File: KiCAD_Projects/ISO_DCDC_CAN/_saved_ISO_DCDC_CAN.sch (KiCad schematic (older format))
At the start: 116 parts, among them IC1 PC817, IC2 PC817, IC3 PC817, IC4 PC817, IC5 PC817, P1 CONN_01X01, P10 CONN_01X02, P11 CONN_01X02, P12 CONN_01X01, P13 CONN_01X04, P14 CONN_01X02, P15 CONN_01X02, P16 TST, P17 CONN_01X06, P19 CONN_01X01, P2 CONN_01X01, P20 CONN_01X01, P21 CONN_01X02, P22 CONN_01X01, P23 CONN_01X01, P25 CONN_01X01, P26 CONN_01X01, P3 CONN_01X01, P4 CONN_01X02, P5 CONN_01X02, P6 CONN_01X04, P7 CONN_01X04, P8 CONN_01X01, P9 CONN_01X01, Q1 MOSFET_N, U1 V23076-D3001-D142, U2 V23076-D3001-D142, U3 V23076-D3001-D142, U4 NCP1117ST285T3G, U5 STM32F103_48, U6 ADM3054, U7 ACS758, U8 ACS758, X1 CRYSTAL

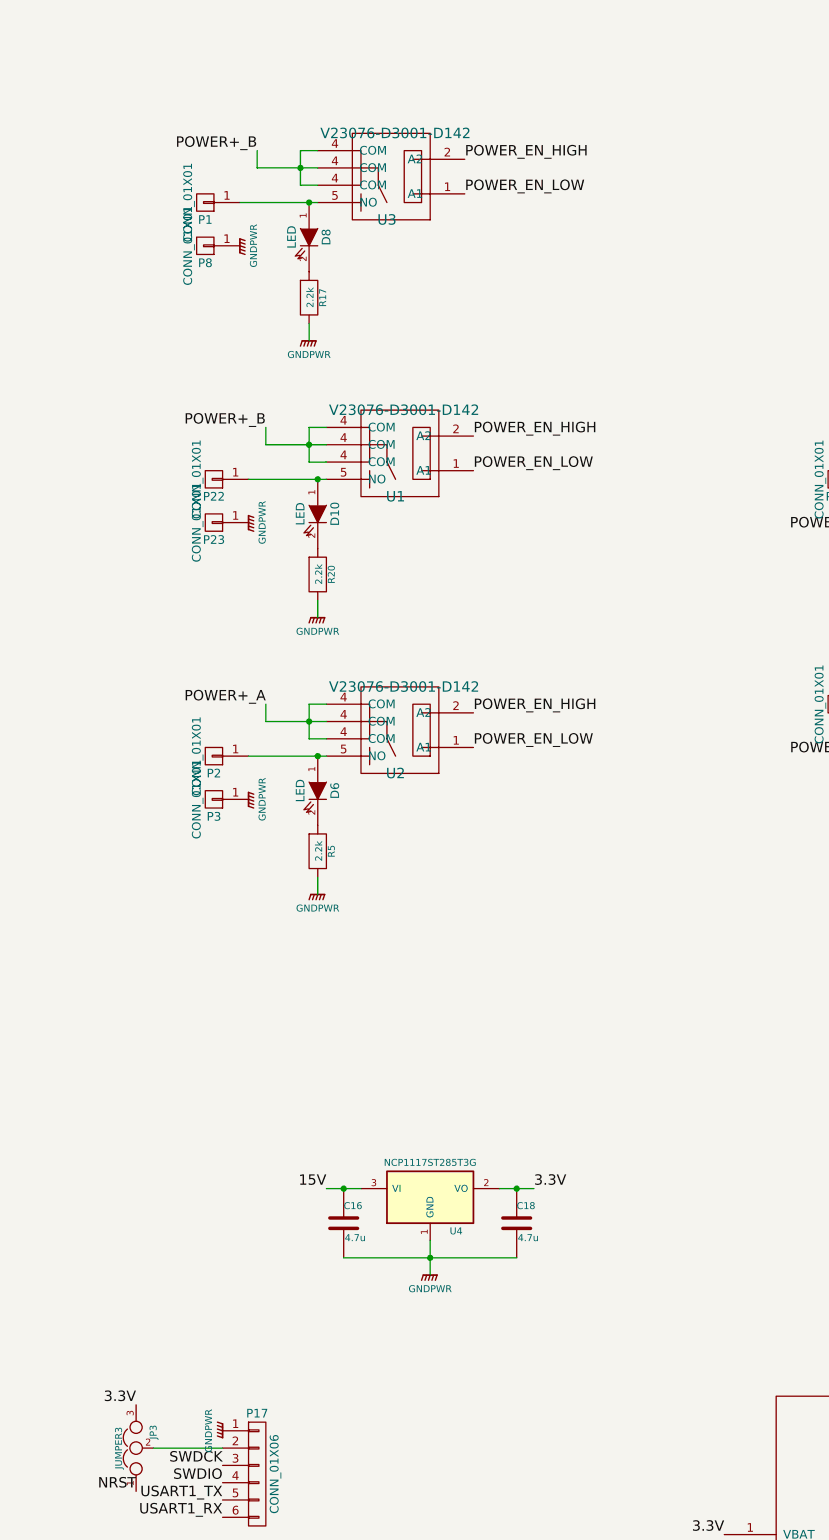
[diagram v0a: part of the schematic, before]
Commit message: 4.0発注かけた｡テレメトリとコンパネ作る
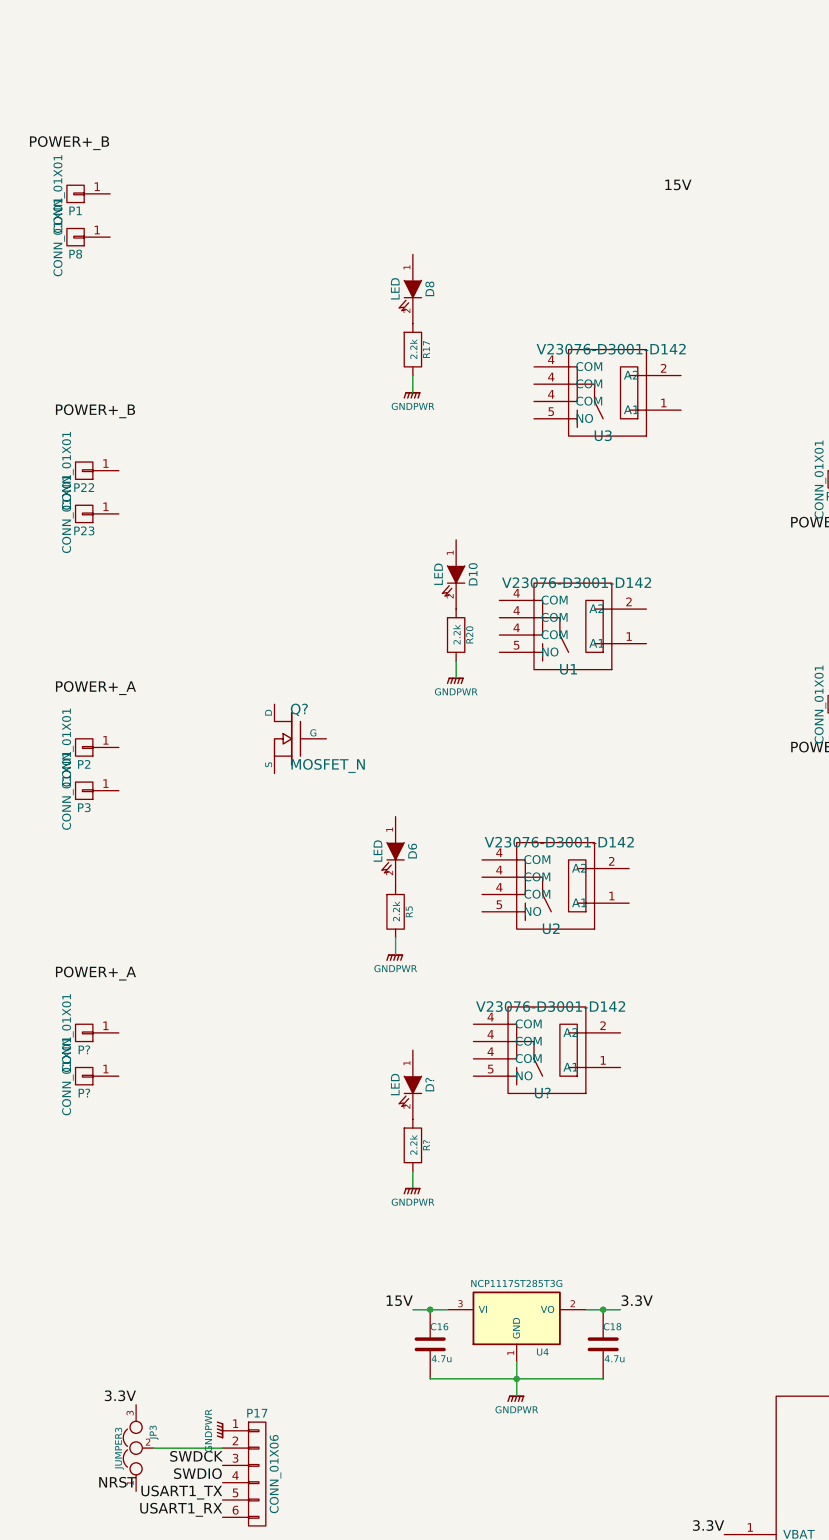
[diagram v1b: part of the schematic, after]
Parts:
- added D?: LED, LEDs:LED_0603, symbol LED
- added P? (x2): CONN_01X01, Connect:1pin, symbol CONN_01X01
- added Q?: MOSFET_N, symbol MOSFET_N
- added R?: 2.2k, RP_KiCAD_Libs:C1608_WP, symbol R
- added U?: V23076-D3001-D142, Relays_ThroughHole:V23076-A3001-D142, symbol V23076-D3001-D142
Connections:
- wire segments 146 -> 129
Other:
- moved on the sheet: C16, C18, D10, D6, D8, P1, P2, P22, P23, P3, P8, R17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
